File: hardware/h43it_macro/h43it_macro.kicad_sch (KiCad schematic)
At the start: 49 parts, among them J1 Conn_01x04_Pin, SW2 SW_Push, U4 ATtiny816-S

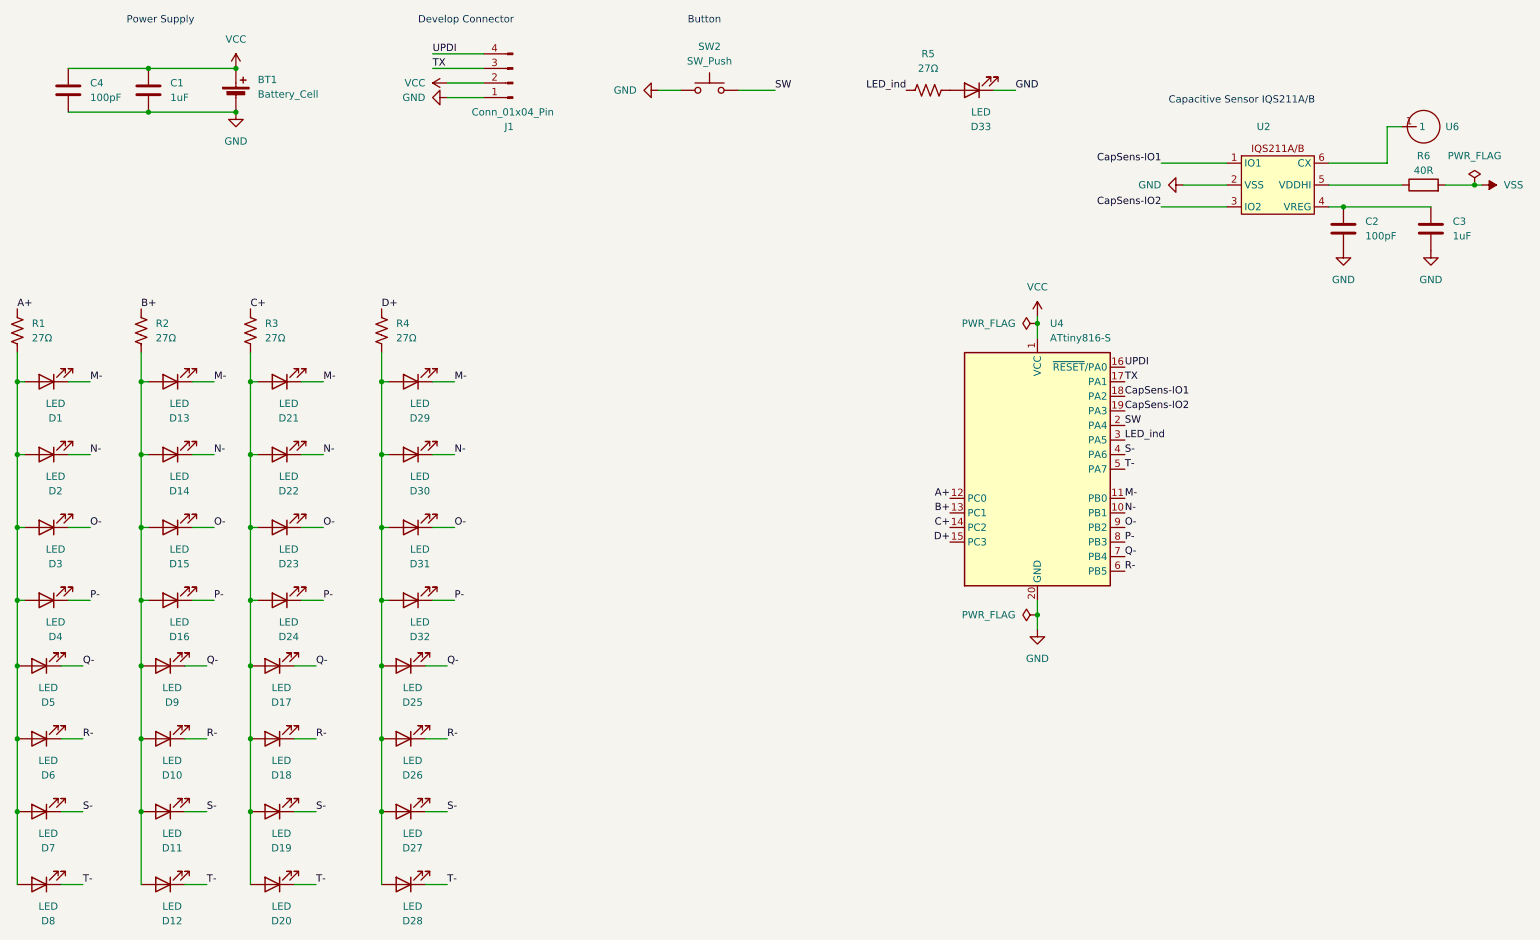
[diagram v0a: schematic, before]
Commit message: pcb for macro
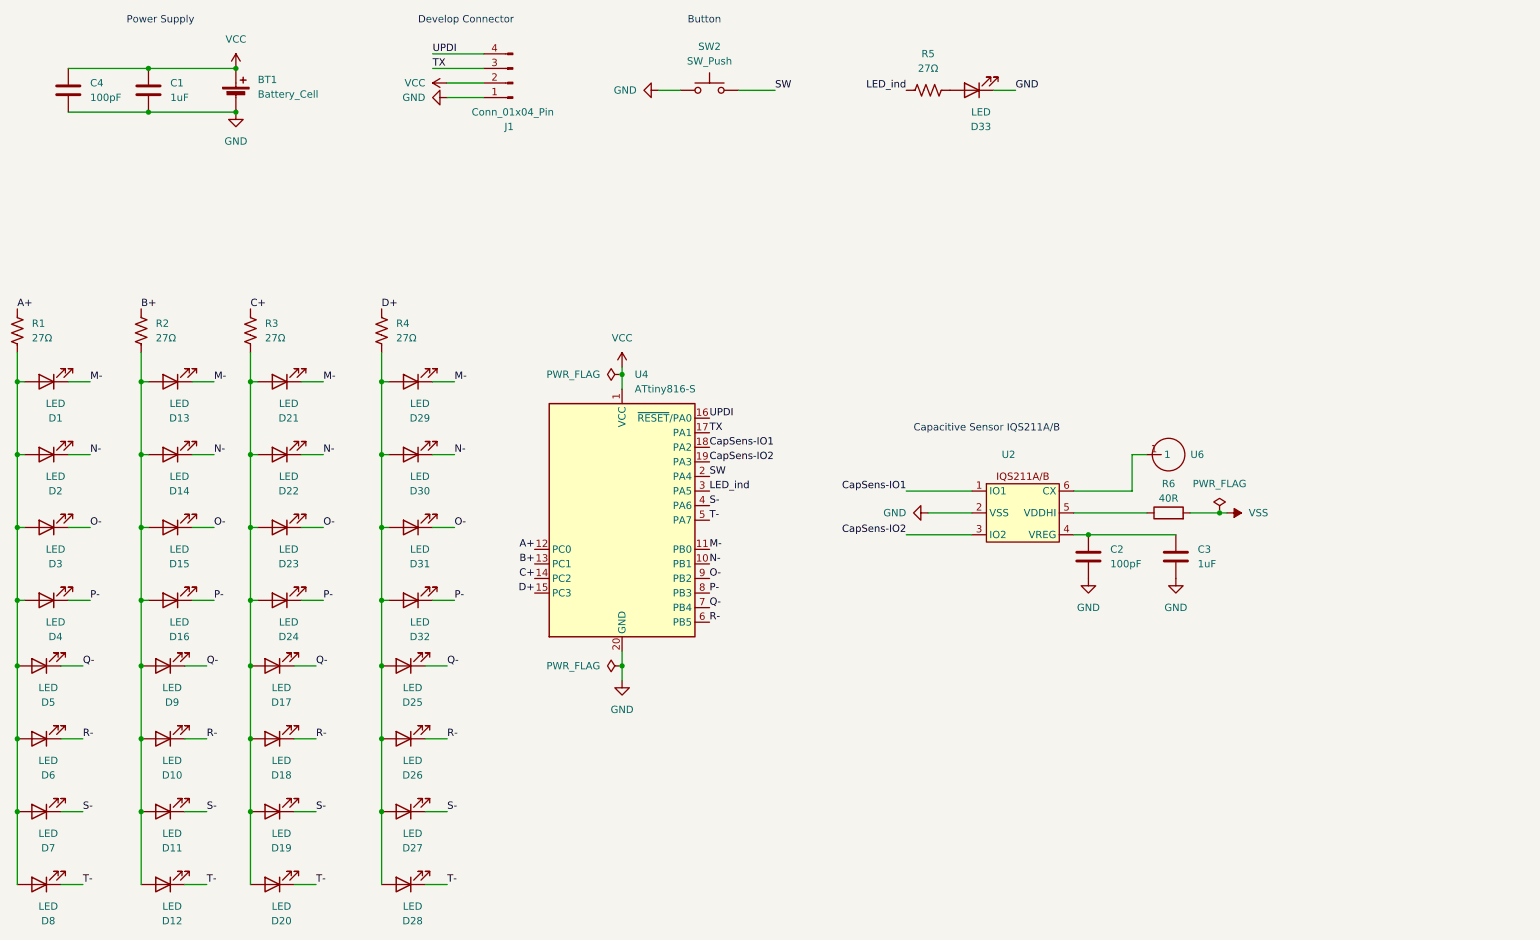
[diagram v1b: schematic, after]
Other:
- moved on the sheet: C2, C3, R6, U2, U4, U6
